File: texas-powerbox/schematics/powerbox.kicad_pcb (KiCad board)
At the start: 2 copper layers, 32 parts, among them J1 BATTERY, J2 ADAPTER, J3 USB_STACKED, J4 USB_STACKED, K1 J107F1CS1224VDC.36, Q1 AOD417, U1 TPS54331GDR

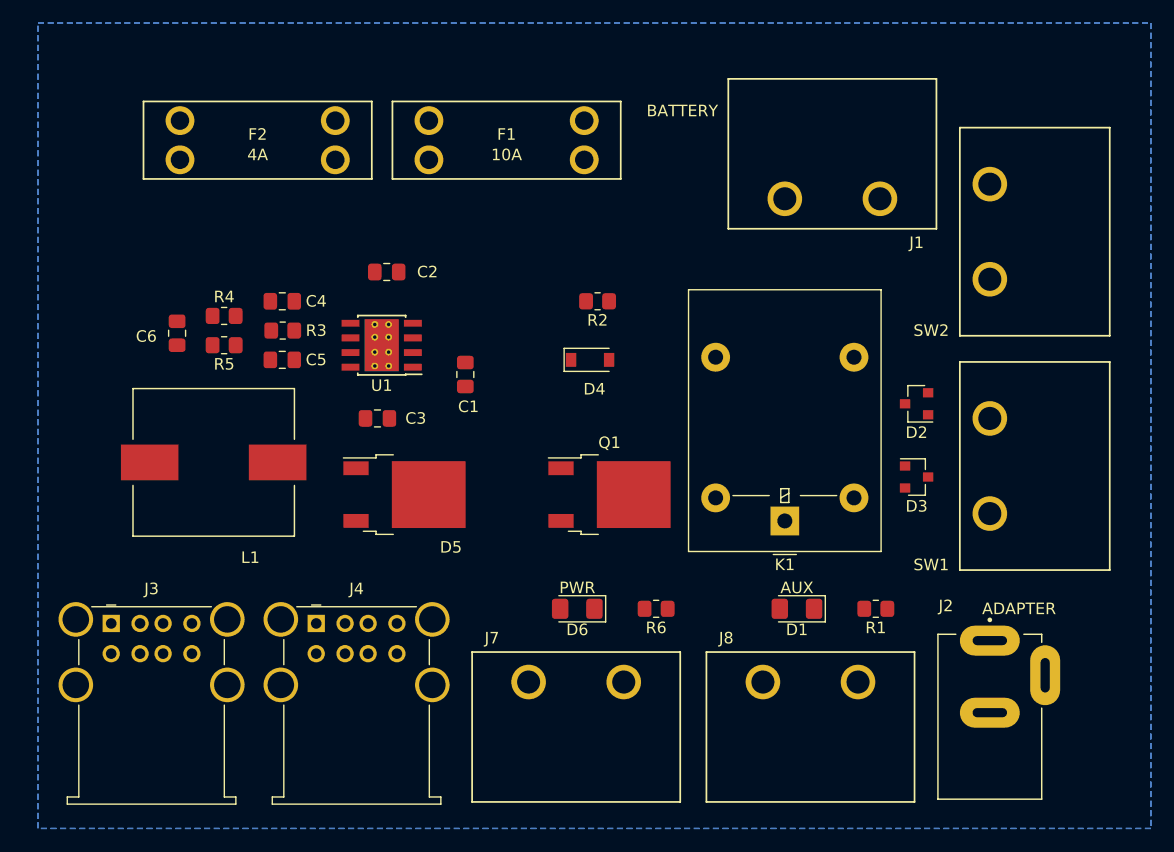
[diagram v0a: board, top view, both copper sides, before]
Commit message: routing
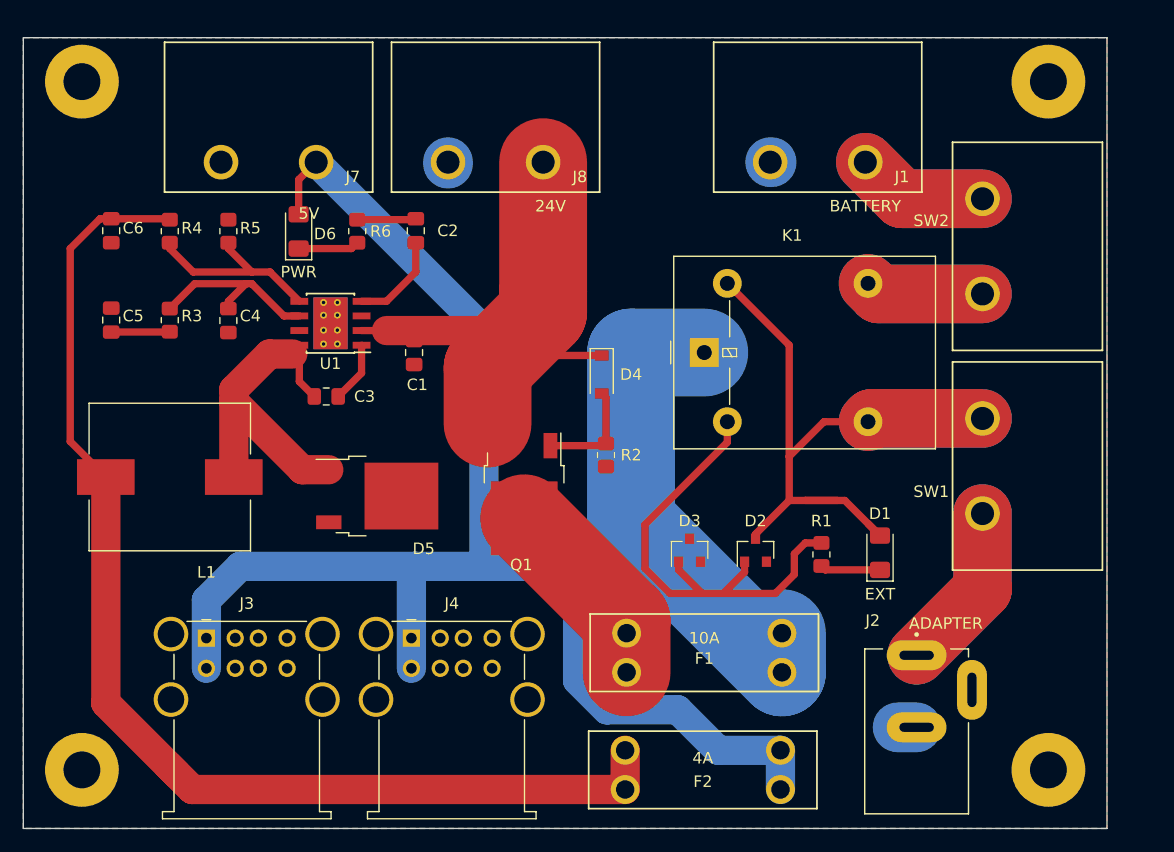
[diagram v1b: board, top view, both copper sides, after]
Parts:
- added REF**: MountingHole_3.2mm_M3_Pad, MountingHole:MountingHole_3.2mm_M3_Pad, F.Cu at (111.8, 95.2)
- added REF**: MountingHole_3.2mm_M3_Pad, MountingHole:MountingHole_3.2mm_M3_Pad, F.Cu at (111.8, 154.9)
- added REF**: MountingHole_3.2mm_M3_Pad, MountingHole:MountingHole_3.2mm_M3_Pad, F.Cu at (195.6, 154.9)
- added REF**: MountingHole_3.2mm_M3_Pad, MountingHole:MountingHole_3.2mm_M3_Pad, F.Cu at (195.6, 95.2)
- D1: value AUX -> EXT
- J7: value ~ -> 5V
- J8: value ~ -> 24V
- moved F2 66.9 mm to (165.6, 154.9), turned to 0 degrees
- moved J8 57.4 mm to (143.5, 102.2), turned to 0 degrees
- moved J7 57.0 mm to (123.8, 102.2), turned to 0 degrees
- moved F1 47.6 mm to (165.7, 144.8), turned to 0 degrees
- moved R6 41.8 mm to (135.6, 108.2), turned to 90 degrees
- moved D6 40.7 mm to (130.6, 108.2), turned to 90 degrees
- moved D3 20.7 mm to (164.5, 135.9), turned to 90 degrees
- moved D2 18.9 mm to (170.2, 135.9), turned to 90 degrees
- moved K1 16.2 mm to (165.7, 118.7), turned to 90 degrees
- moved C5 15.2 mm to (114.3, 115.9), turned to 90 degrees
- moved R2 13.4 mm to (157.2, 127.6), turned to 270 degrees
- moved C6 10.6 mm to (114.3, 108.2)
- moved R5 9.90 mm to (124.5, 108.2), turned to 90 degrees
- moved R3 9.84 mm to (119.4, 115.9), turned to 90 degrees
- moved R4 8.73 mm to (119.4, 108.2), turned to 270 degrees
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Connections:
- F1 pad 1: GND -> Net-(F1-Pad1)
- J1 pad 1: Net-(F1-Pad2) -> GND
- J2 pad 2: Net-(F1-Pad2) -> GND
- K1 pad 1: Net-(K1-Pad1) -> Net-(F1-Pad1)
- Q1 pad 2: Net-(K1-Pad1) -> Net-(F1-Pad2)
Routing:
- net +5V: track 0.00 -> 126.7 mm
- net Net-(C6-Pad1): track 0.00 -> 113.7 mm
- net Net-(D1-Pad2): track 0.00 -> 67.2 mm
- net +24V: track 0.00 -> 46.4 mm
- net Net-(F1-Pad1): track 0.00 -> 42.9 mm
- net Net-(D2-Pad2): track 0.00 -> 41.8 mm
- net Net-(C3-Pad1): track 0.00 -> 29.7 mm
- net Net-(J2-Pad1): track 0.00 -> 29.3 mm
- net Net-(J1-Pad2): track 0.00 -> 23.0 mm
- net Net-(K1-Pad4): track 0.00 -> 20.6 mm
- net Net-(F1-Pad2): track 0.00 -> 17.0 mm
- net Net-(R4-Pad2): track 0.00 -> 17.0 mm
- net Net-(C4-Pad1): track 0.00 -> 16.1 mm
- net Net-(D4-Pad2): track 0.00 -> 9.38 mm
- net Net-(C2-Pad1): track 0.00 -> 8.29 mm
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- added copper zone on F.Cu, net GND
- removed copper zone on B.Cu, net (none)
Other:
- board outline added: 94 x 68.6 mm
